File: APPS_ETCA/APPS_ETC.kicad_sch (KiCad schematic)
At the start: 21 parts, among them P1 DTM1312PC12PDR008, U1 NSL-32, U2 DK1A1B-12V, U3 MCP6004, U6 LM7805_TO220, U8 LM7809_TO220

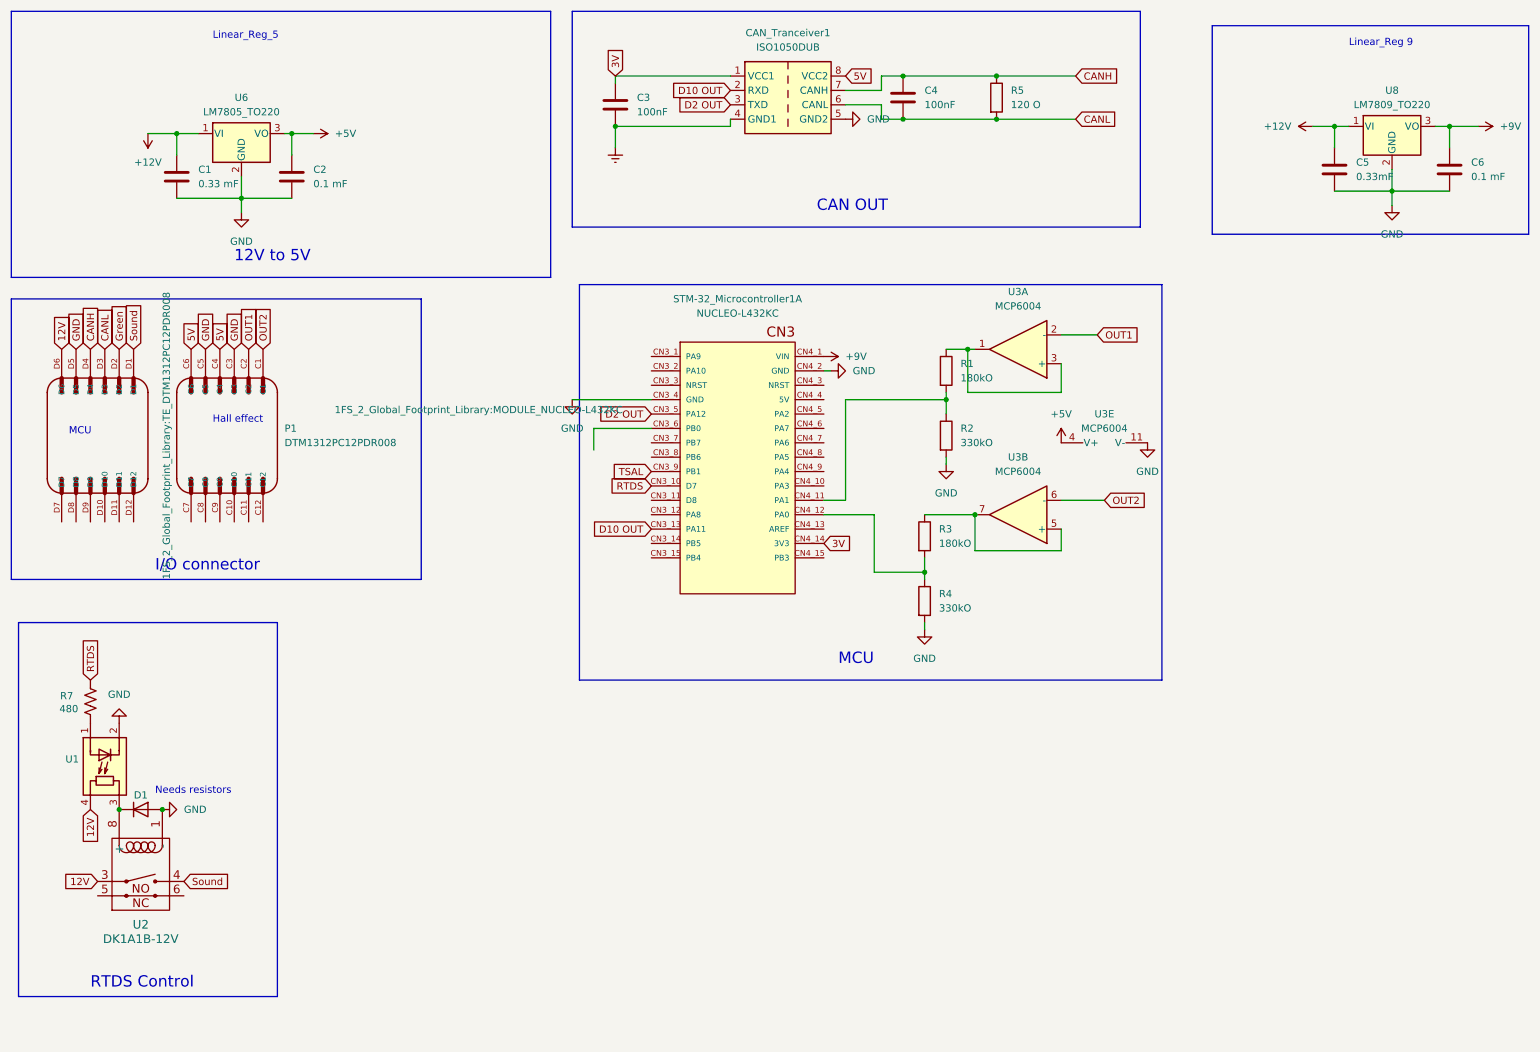
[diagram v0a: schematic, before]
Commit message: updated schema
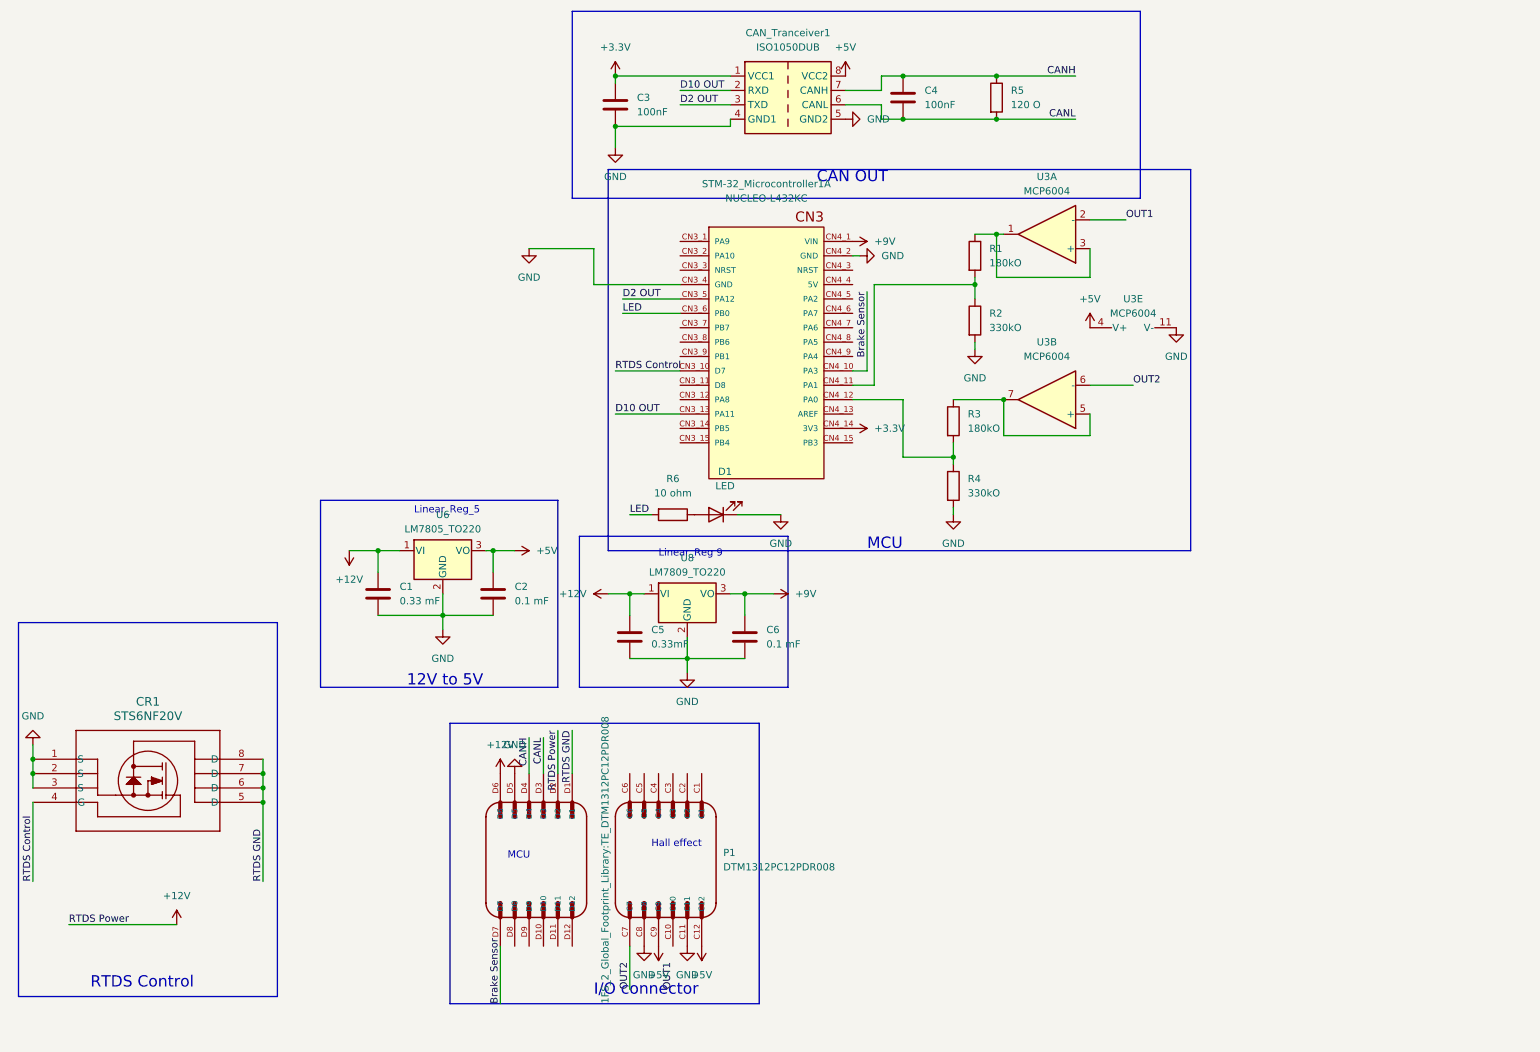
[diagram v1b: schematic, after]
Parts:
- removed D1: D, Diode_THT:D_DO-41_SOD81_P10.16mm_Horizontal, symbol Device:D
- removed R7: 480, Resistor_SMD:R_0805_2012Metric_Pad1.20x1.40mm_HandSolder, symbol Device:R_US
- removed U1: NSL-32, 1FS_2_Global_Footprint_Library:OptoCoupler 6-SOP, symbol Isolator:NSL-32
- removed U2: DK1A1B-12V, 1FS_2_Global_Footprint_Library:RELAY_DK2A_PAN, symbol 2FS-1_Symbol Library:DK1A1B-12V
- added CR1: STS6NF20V, 1FS_2_Global_Footprint_Library:SOIC127P600X175-8N, symbol 1FS_2_Global_Symbol_Library:STS6NF20V
- added D1: LED, LED_THT:LED_D10.0mm, symbol Device:LED
- added R6: 10 ohm, Resistor_SMD:R_0805_2012Metric_Pad1.20x1.40mm_HandSolder, symbol Device:R
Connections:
- net 12V is gone; now on net +12V: P1.D6
- net Earth is gone; now on net GND: C3.2, CAN_Tranceiver1.4 (GND1)
- net Green is gone; now on net +12V: P1.D2
- net +5V: now also CAN_Tranceiver1.8 (VCC2), P1.C12, P1.C9
- net GND: now also P1.C11, P1.C8, CR1.1 (S), CR1.2 (S), CR1.3 (S), D1.1 (K); no longer P1.C3, P1.C5
- net OUT1: no longer P1.C2
- net OUT2: now also P1.C7; no longer P1.C1
- net Brake Sensor: now reaches P1.D7
- net Brake Sensor: now also STM-32_Microcontroller1.CN4_10 (PA3)
- net LED: now reaches STM-32_Microcontroller1.CN3_6 (PB0)
- net LED: now also R6.2
- net 3V renamed +3.3V
- removed net 5V: CAN_Tranceiver1.8 (VCC2), P1.C4, P1.C6
- net RTDS renamed RTDS Control
- net RTDS Control: now also CR1.4 (G)
- net Sound renamed RTDS GND
- net RTDS GND: now also CR1.5 (D), CR1.6 (D), CR1.7 (D), CR1.8 (D)
- net TSAL: no longer names the net of STM-32_Microcontroller1.CN3_9 (PB1)
- new net: D1.2 (A), R6.1
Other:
- note removed: "Needs resistors"
- moved on the sheet: C1, C2, C5, C6, P1, R1, R2, R3, R4, STM-32_Microcontroller1A, U3A, U3B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
